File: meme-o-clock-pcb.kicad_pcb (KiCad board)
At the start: 4 copper layers, 88 x 100 mm, 24 parts, among them J1 USB_C_Receptacle_USB2.0_16P, J2 Conn_01x04_Pin, J3 Conn_01x02_Pin, J4 Conn_01x03_Pin, SW1 SW_Push, SW2 SW_Push, SW3 SW_Push, SW4 SW_Push, U1 MAX98357A, U2 APDS-9306

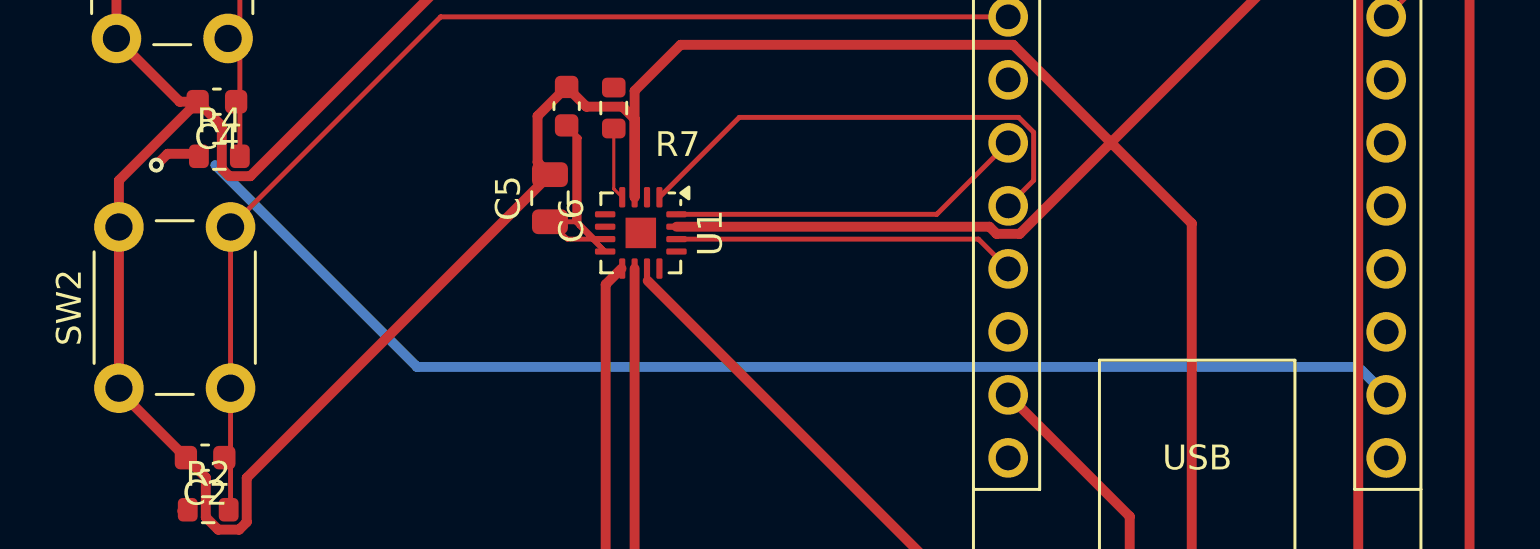
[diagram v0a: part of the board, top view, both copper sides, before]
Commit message: Autosave
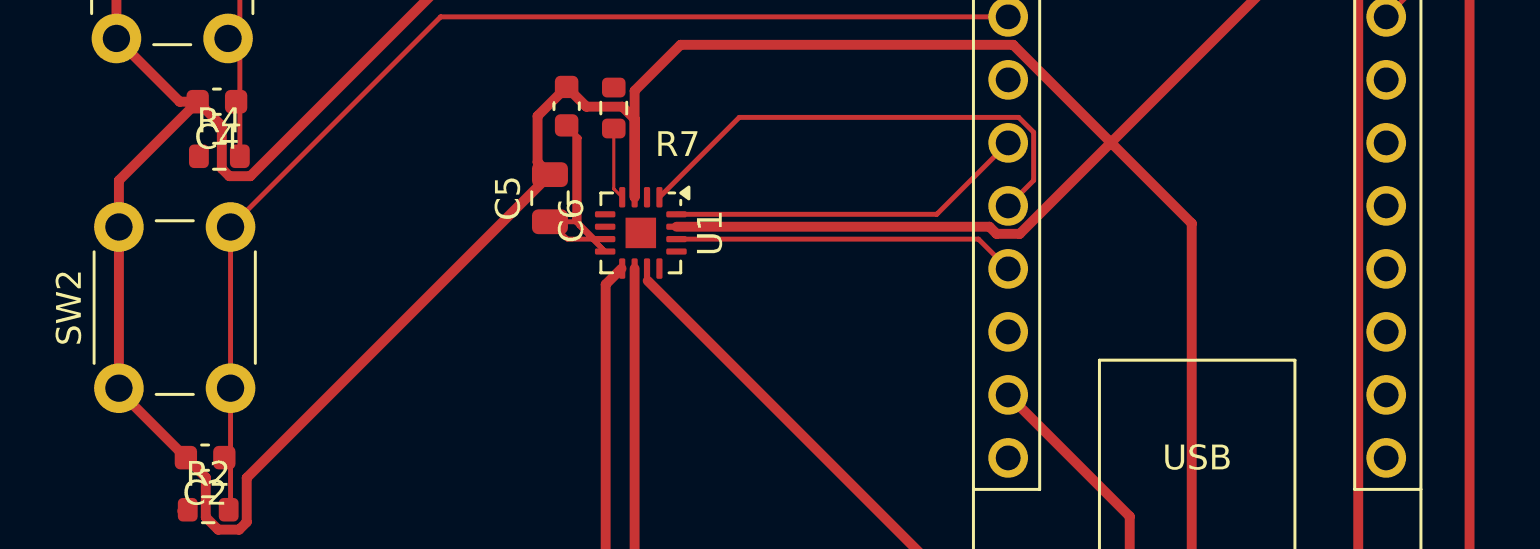
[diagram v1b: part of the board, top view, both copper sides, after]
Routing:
- net +3V3: track 53.2 -> 0.25 mm, vias 1 -> 0
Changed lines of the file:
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@@
-	)
-	(segment
-		(start 79.611712 99.3)
-		(end 79.155856 99.755856)
-		(width 0.4)
-		(layer "F.Cu")
-		(net "+3V3")
-	)
-	(segment
-		(start 80.8 99.4)
-		(end 80.7 99.3)
-		(width 0.4)
-		(layer "F.Cu")
-		(net "+3V3")
-	)
-	(segment
-		(start 80.875 99.4)
-		(end 80.8 99.4)
-		(width 0.4)
-		(layer "F.Cu")
-		(net "+3V3")
-	)
-	(segment
-		(start 80.7 99.3)
-		(end 79.611712 99.3)
-		(width 0.4)
-		(layer "F.Cu")
-		(net "+3V3")
-	)
-	(via
-		(at 79.155856 99.755856)
-		(size 0.6)
-		(drill 0.3)
-		(layers "F.Cu" "B.Cu")
-		(net "+3V3")
-	)
-	(segment
-		(start 127.613 107.893)
-		(end 128.74 109.02)
-		(width 0.4)
-		(layer "B.Cu")
-		(net "+3V3")
-	)
-	(segment
-		(start 89.669662 107.893)
-		(end 127.613 107.893)
-		(width 0.4)
-		(layer "B.Cu")
-		(net "+3V3")
-	)
-	(segment
-		(start 81.532518 99.755856)
-		(end 89.669662 107.893)
-		(width 0.4)
-		(layer "B.Cu")
-		(net "+3V3")
 	)
 	(segment
